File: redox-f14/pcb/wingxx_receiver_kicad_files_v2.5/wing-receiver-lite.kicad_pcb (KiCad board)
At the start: 2 copper layers, 22.6 x 43.9 mm, 27 parts, among them U1 ATmega32U4-AU, X1 Crystal_GND24

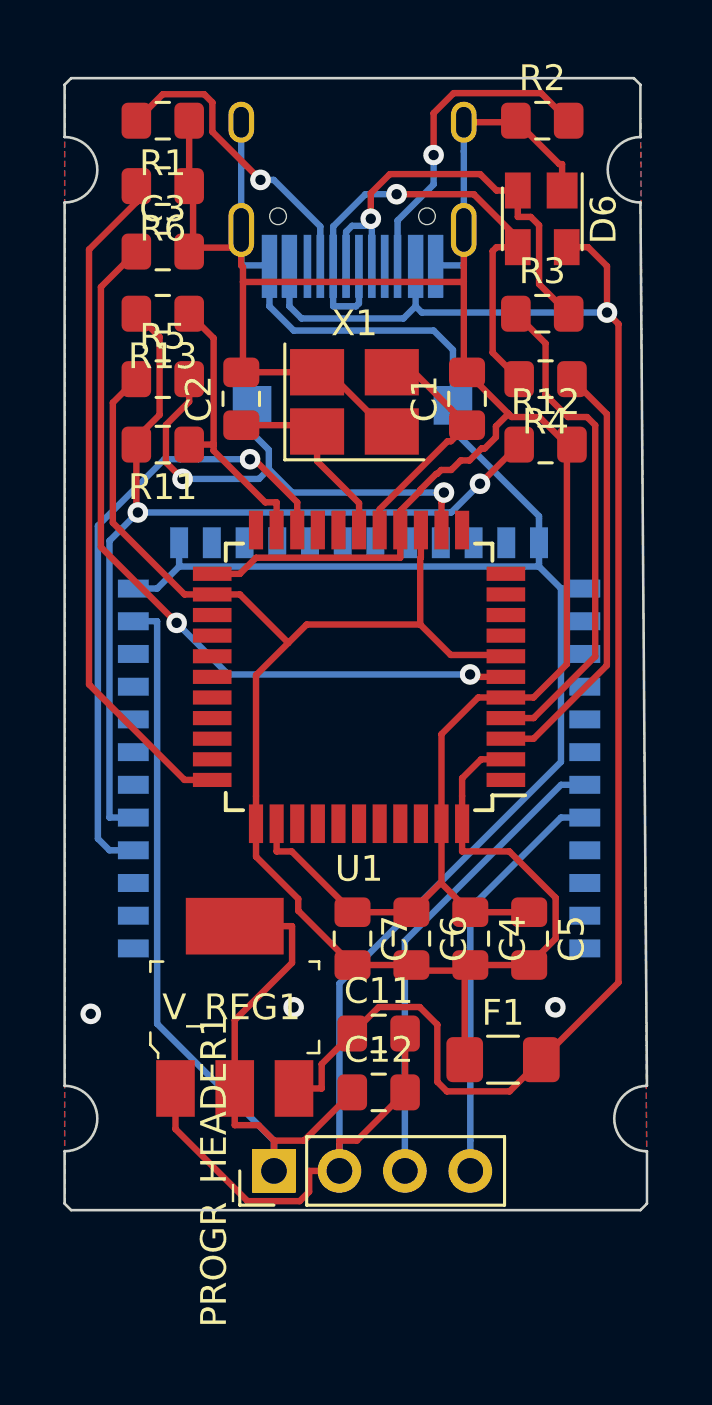
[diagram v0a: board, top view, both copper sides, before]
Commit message: new receiver
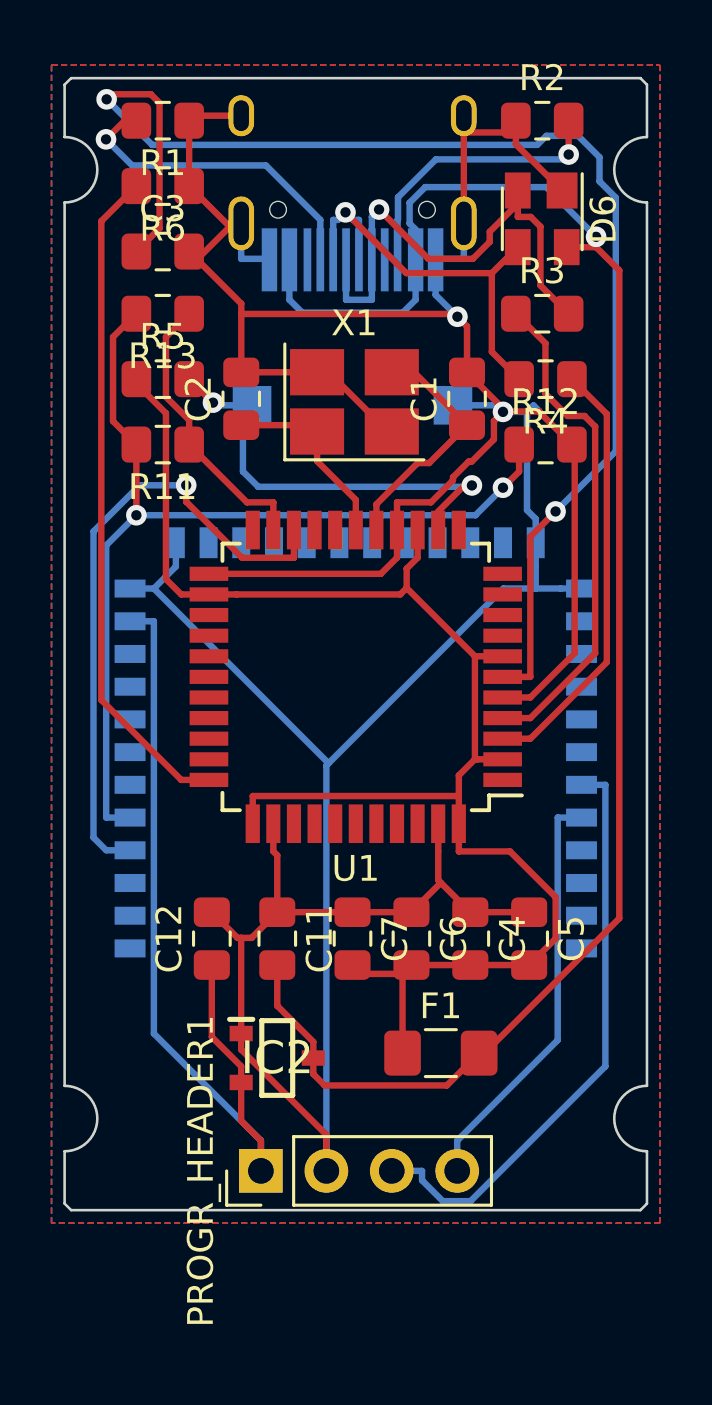
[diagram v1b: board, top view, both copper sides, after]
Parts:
- removed V_REG1: LD1117S33CTR, redox_w_receiver_footprints:SOT-223
- added IC2: XC6206P332MR, XC6206P332MR:SOT95P280X130-3N, F.Cu at (76.8, 131.0)
- C11, C12: value 10uF -> 1uF
- moved C12 8.81 mm to (74.3, 126.4), turned to 90 degrees
- moved C11 5.39 mm to (76.8, 126.4), turned to 270 degrees
- moved F1 2.43 mm to (83.2, 130.8)
- moved PROGR_HEADER1 0.51 mm to (76.2, 135.4)
- moved USB1 0.25 mm to (79.8, 91.8)
- moved U1 0.13 mm to (79.9, 116.2)
- moved nrf1 0.13 mm to (78.0, 111.0)
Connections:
- C11 pad 1: VCC -> GND
- C11 pad 2: GND -> VCC
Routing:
- net GND: track 187.6 -> 164.3 mm, vias 3 -> 2
- net Net-(C3-Pad1): track 29.9 -> 51.7 mm
- net +3.3V: track 41.8 -> 32.8 mm
- net SWDIO: track 18.4 -> 23.0 mm
- net +5V: track 65.0 -> 60.9 mm
- net Net-(D6-Pad3): track 20.8 -> 17.0 mm
- net Net-(R5-Pad2): track 19.4 -> 17.0 mm
- net Net-(D6-Pad2): track 17.4 -> 19.4 mm
- net VCC: track 64.6 -> 66.5 mm
- net Net-(R2-Pad2): track 12.5 -> 11.1 mm
- net Net-(R1-Pad2): track 11.9 -> 12.6 mm
- net TXODIV: track 37.6 -> 38.3 mm
- added copper zone on B.Cu, net (none)
- added copper zone on F.Cu, net (none)
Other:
- outline, holes or cut-outs redrawn
